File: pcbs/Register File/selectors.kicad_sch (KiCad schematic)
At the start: 1 part, among them U1001 74HC138

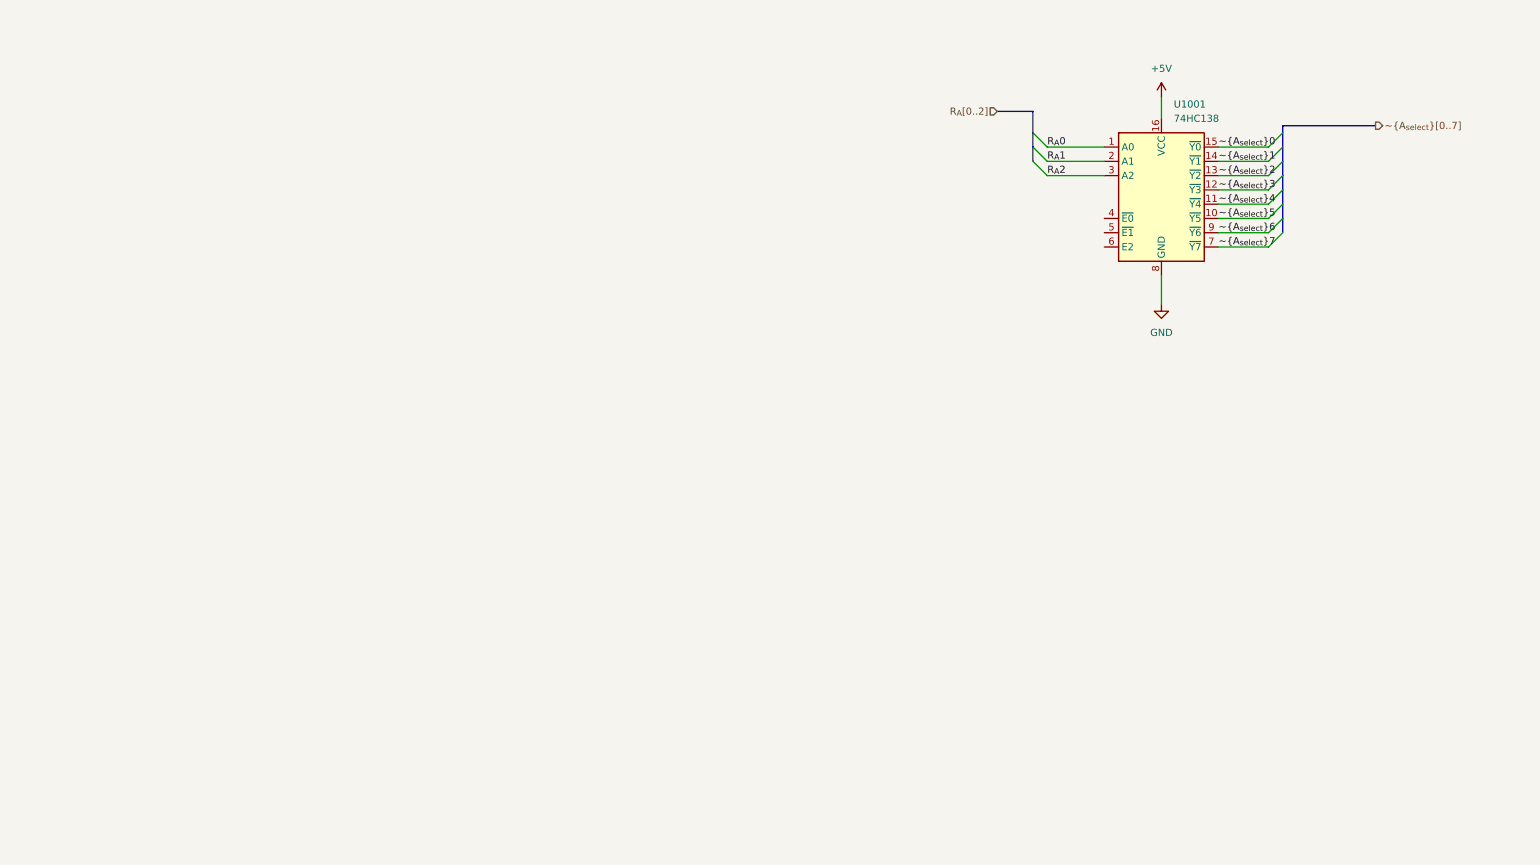
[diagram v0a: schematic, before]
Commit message: More work
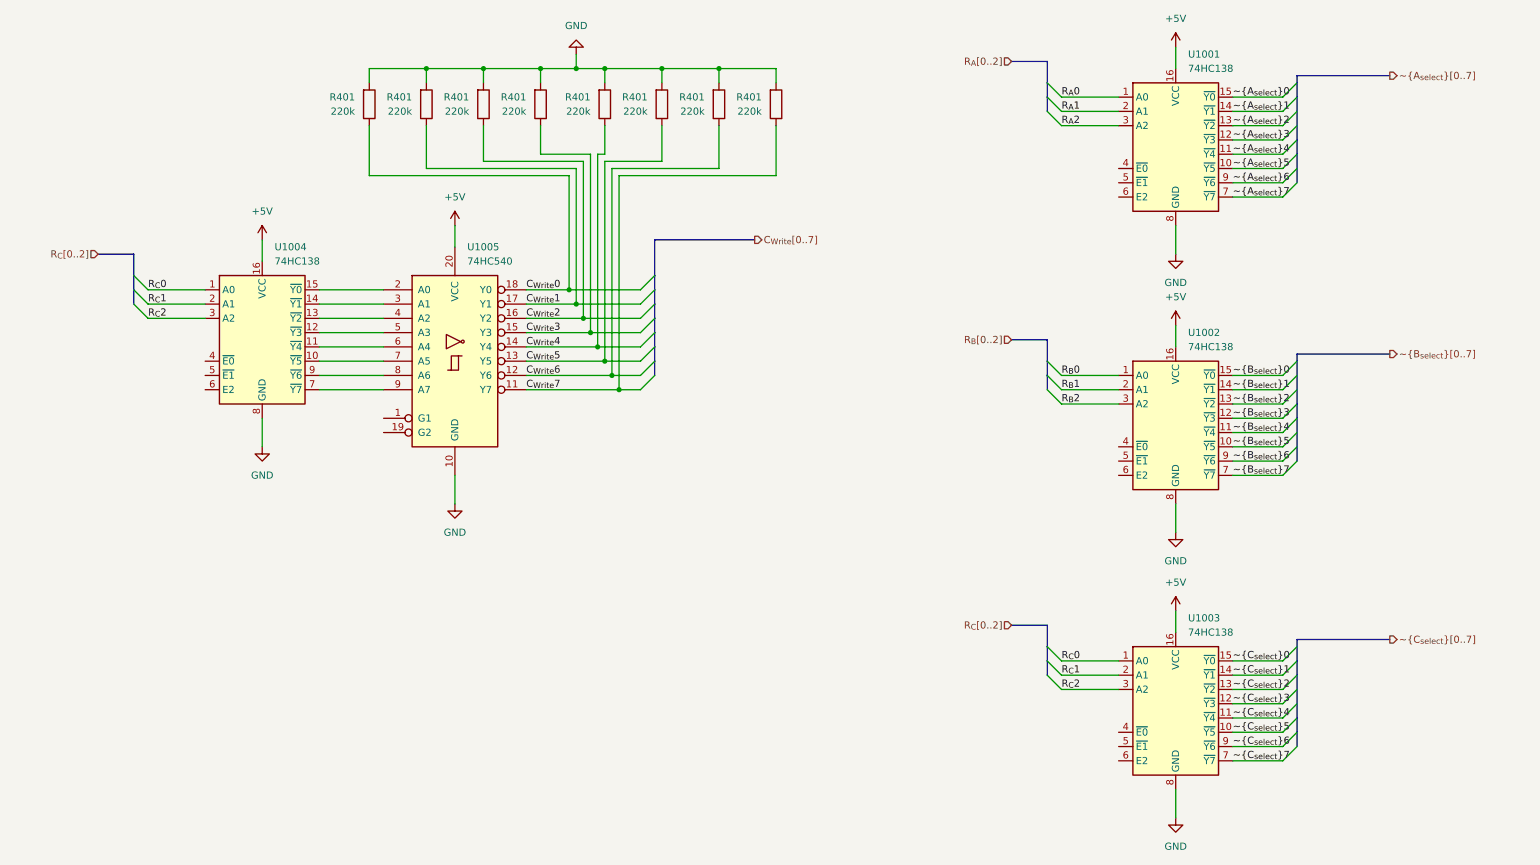
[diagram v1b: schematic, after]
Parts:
- added R401 (x8): 220k, Resistor_SMD:R_0603_1608Metric, symbol Device:R
- added U1002, U1003, U1004: 74HC138, Package_DIP:DIP-16_W7.62mm_Socket, symbol 74xx:74HC138
- added U1005: 74HC540, Package_DIP:DIP-20_W7.62mm_Socket, symbol 74xx:74LS540
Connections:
- net +5V: now also U1002.16 (VCC), U1003.16 (VCC), U1004.16 (VCC), U1005.20 (VCC)
- net GND: now also R401.2, R401.2, R401.2, R401.2, R401.2, R401.2, R401.2, R401.2, U1002.8 (GND), U1003.8 (GND), U1004.8 (GND), U1005.10 (GND)
- new net: U1004.15 (~{Y0}), U1005.2 (A0)
- new net: U1004.14 (~{Y1}), U1005.3 (A1)
- new net: U1004.13 (~{Y2}), U1005.4 (A2)
- new net: U1004.12 (~{Y3}), U1005.5 (A3)
- new net: U1004.11 (~{Y4}), U1005.6 (A4)
- new net: U1004.10 (~{Y5}), U1005.7 (A5)
- new net: U1004.9 (~{Y6}), U1005.8 (A6)
- new net: U1004.7 (~{Y7}), U1005.9 (A7)
- new net C_{Write}0: R401.1, U1005.18 (Y0)
- new net C_{Write}1: R401.1, U1005.17 (Y1)
- new net C_{Write}2: R401.1, U1005.16 (Y2)
- new net C_{Write}3: R401.1, U1005.15 (Y3)
- new net C_{Write}4: R401.1, U1005.14 (Y4)
- new net C_{Write}5: R401.1, U1005.13 (Y5)
- new net C_{Write}6: R401.1, U1005.12 (Y6)
- new net C_{Write}7: R401.1, U1005.11 (Y7)
- new net R_{B}0: U1002.1 (A0)
- new net R_{B}1: U1002.2 (A1)
- new net R_{B}2: U1002.3 (A2)
- new net R_{C}0: U1003.1 (A0), U1004.1 (A0)
- new net R_{C}1: U1003.2 (A1), U1004.2 (A1)
- new net R_{C}2: U1003.3 (A2), U1004.3 (A2)
- new net ~{B_{select}}0: U1002.15 (~{Y0})
- new net ~{B_{select}}1: U1002.14 (~{Y1})
- new net ~{B_{select}}2: U1002.13 (~{Y2})
- new net ~{B_{select}}3: U1002.12 (~{Y3})
- new net ~{B_{select}}4: U1002.11 (~{Y4})
- new net ~{B_{select}}5: U1002.10 (~{Y5})
- new net ~{B_{select}}6: U1002.9 (~{Y6})
- new net ~{B_{select}}7: U1002.7 (~{Y7})
- new net ~{C_{select}}0: U1003.15 (~{Y0})
- new net ~{C_{select}}1: U1003.14 (~{Y1})
- new net ~{C_{select}}2: U1003.13 (~{Y2})
- new net ~{C_{select}}3: U1003.12 (~{Y3})
- new net ~{C_{select}}4: U1003.11 (~{Y4})
- new net ~{C_{select}}5: U1003.10 (~{Y5})
- new net ~{C_{select}}6: U1003.9 (~{Y6})
- new net ~{C_{select}}7: U1003.7 (~{Y7})
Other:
- moved on the sheet: U1001
